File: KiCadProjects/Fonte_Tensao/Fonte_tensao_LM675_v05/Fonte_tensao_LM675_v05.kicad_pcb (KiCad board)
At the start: 2 copper layers, 90 x 100 mm, 33 parts, among them J1 alimentacao analogica, J2 sinais analogicos, J3 comunicacao / sinais digitais, J4 Barrel_Jack, U1 L7809, U2 LM7909_TO220, U3 LM675, U4 L7805, U5 L7905, U6 LM1117T-3.3

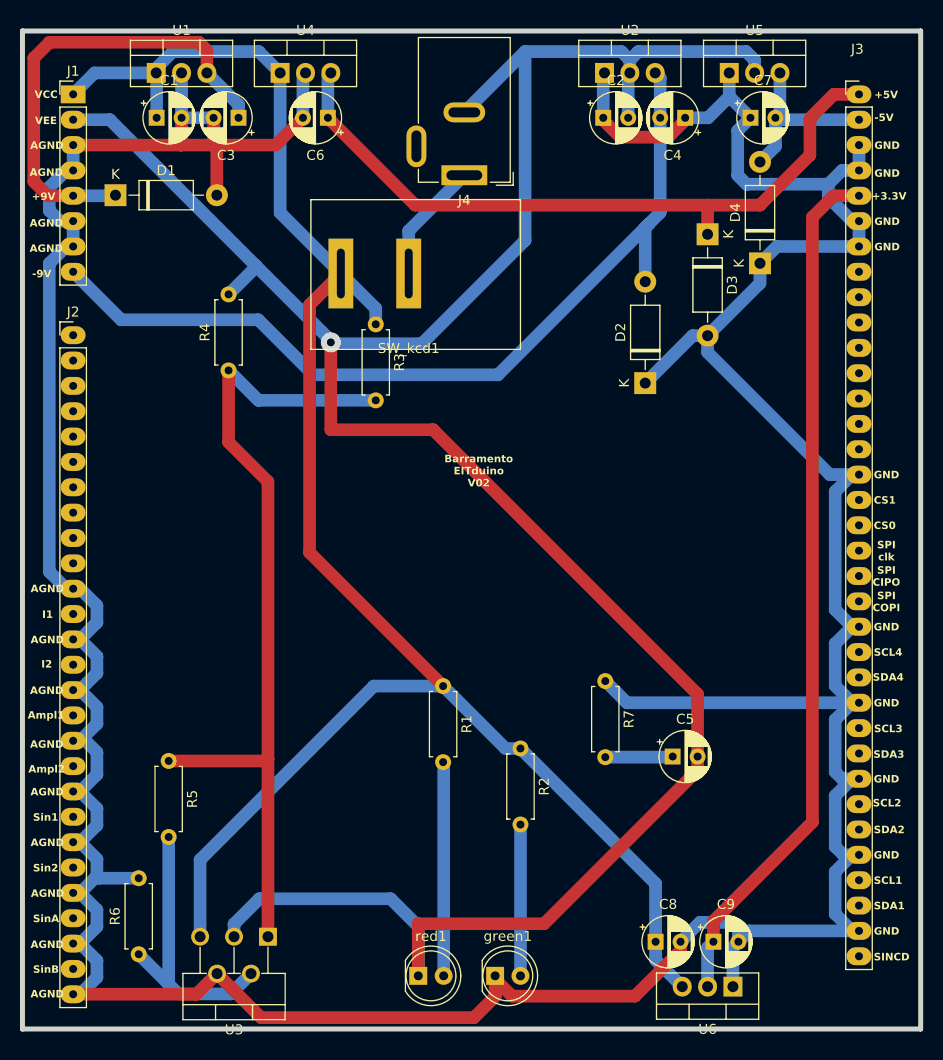
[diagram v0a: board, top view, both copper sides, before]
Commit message: versao para fabricacao jlcpcb revisao Gustavo
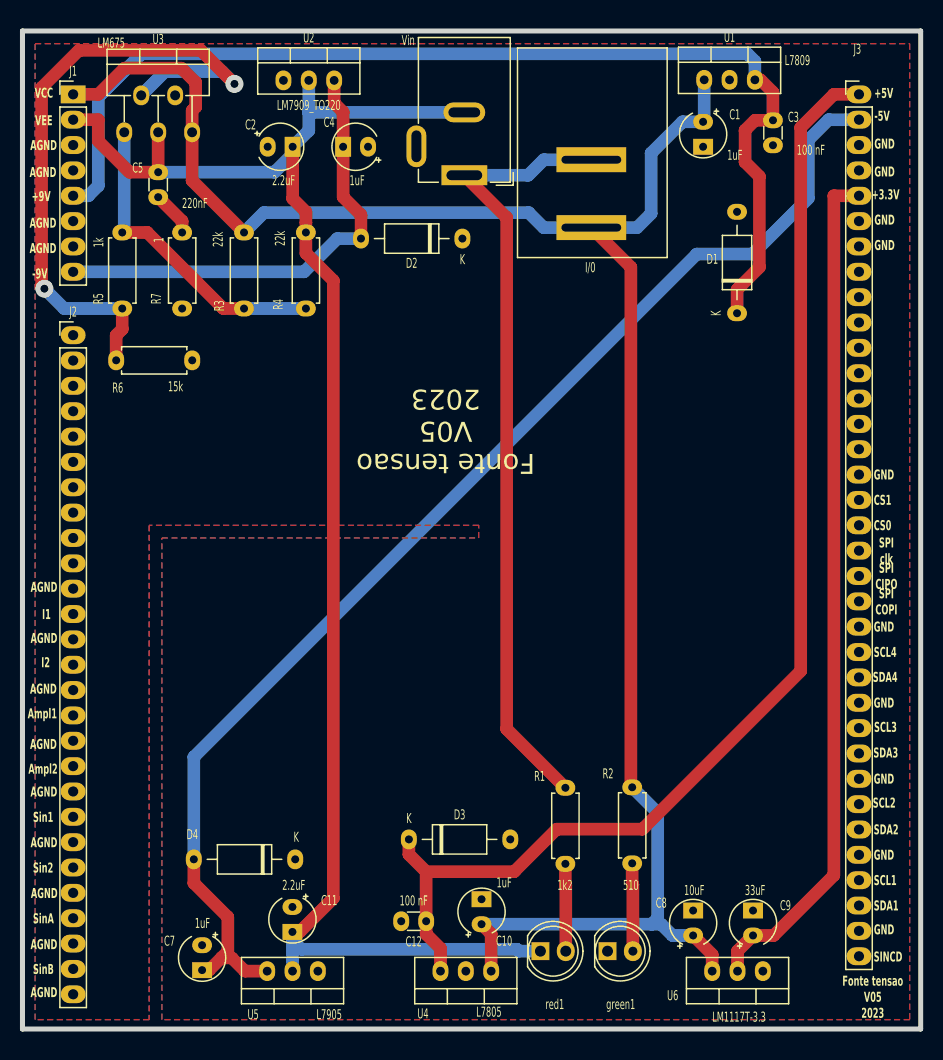
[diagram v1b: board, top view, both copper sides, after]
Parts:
- removed C6: 1uF, Capacitor_THT:CP_Radial_D5.0mm_P2.50mm
- added C10: 1uF, Capacitor_THT:CP_Radial_Tantal_D4.5mm_P2.50mm, F.Cu at (147.6, 140.3)
- added C11: 2.2uF, Capacitor_THT:CP_Radial_Tantal_D4.5mm_P2.50mm, F.Cu at (128.7, 138.6)
- added C12: 100 nF, Capacitor_THT:C_Disc_D3.0mm_W1.6mm_P2.50mm, F.Cu at (142.1, 140.0)
- C1: value 3.3uF -> 1uF; footprint Capacitor_THT:CP_Radial_D5.0mm_P2.50mm -> Capacitor_THT:CP_Radial_Tantal_D4.5mm_P2.50mm
- C2: value 22uF -> 2.2uF; footprint Capacitor_THT:CP_Radial_D5.0mm_P2.50mm -> Capacitor_THT:CP_Radial_Tantal_D4.5mm_P2.50mm
- C3: value 1uF -> 100 nF; footprint Capacitor_THT:CP_Radial_D5.0mm_P2.50mm -> Capacitor_THT:C_Disc_D3.0mm_W1.6mm_P2.50mm
- C4, C7: footprint Capacitor_THT:CP_Radial_D5.0mm_P2.50mm -> Capacitor_THT:CP_Radial_Tantal_D4.5mm_P2.50mm
- C5: value 2.2uF -> 220nF; footprint Capacitor_THT:CP_Radial_D5.0mm_P2.50mm -> Capacitor_THT:C_Disc_D3.0mm_W1.6mm_P2.50mm
- C8: value 100uF -> 10uF; footprint Capacitor_THT:CP_Radial_D5.0mm_P2.50mm -> Capacitor_THT:CP_Radial_Tantal_D4.5mm_P2.50mm
- C9: value 100uF -> 33uF; footprint Capacitor_THT:CP_Radial_D5.0mm_P2.50mm -> Capacitor_THT:CP_Radial_Tantal_D4.5mm_P2.50mm
- I/0: renamed from SW_kcd1; value chave_gangorra_2_pinos -> Vin
- Vin: renamed from J4; value Barrel_Jack -> Vin
- moved C7 99.5 mm to (119.6, 142.4), turned to -90 degrees
- moved U5 99.0 mm to (131.2, 145.0), turned to 180 degrees
- moved U4 92.5 mm to (148.6, 145.0), turned to 180 degrees
- moved U3 81.9 mm to (111.8, 61.0), turned to 0 degrees
- moved C5 76.2 mm to (115.2, 67.5), turned to 90 degrees
- moved D4 75.7 mm to (128.9, 133.8), turned to 180 degrees
- moved D3 67.6 mm to (140.3, 131.8), turned to 0 degrees
- moved D1 63.4 mm to (173.2, 79.1), turned to 90 degrees
- moved R6 59.6 mm to (111.0, 83.8), turned to 0 degrees
- moved R7 56.5 mm to (117.6, 78.6), turned to 90 degrees
- moved U1 54.9 mm to (169.9, 55.7)
- moved C1 54.8 mm to (169.8, 59.9), turned to -90 degrees
- moved C3 53.6 mm to (176.8, 59.8), turned to -90 degrees
- moved R5 53.2 mm to (111.6, 71.0)
- moved C2 33.7 mm to (126.2, 62.4)
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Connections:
- I/0 pad 1: Net-(J4-Pad1) -> Vin
- R1 pad 1: VCC -> Vin
- Vin pad 1: Net-(J4-Pad1) -> Vin
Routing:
- net Earth: track 447.4 -> 0.00 mm
- net -5V: track 18.2 -> 125.9 mm
- net VEE: track 252.2 -> 166.4 mm, vias 1 -> 0
- net Vin: track 0.00 -> 78.9 mm
- net +9V: track 47.6 -> 109.8 mm
- net Net-(U3-+): track 84.4 -> 31.7 mm
- net +5V: track 71.1 -> 122.0 mm
- net -9V: track 90.0 -> 47.2 mm
- net Net-(U3--): track 28.5 -> 67.4 mm, vias 0 -> 2
- net Net-(red1-A): track 21.4 -> 8.77 mm
- net Net-(J4-Pad1): track 12.2 -> 0.00 mm
- net VCC: track 185.7 -> 194.9 mm
- net Net-(green1-A): track 15.2 -> 8.83 mm
- net Net-(C5-Pad1): track 6.77 -> 4.53 mm
- net +3.3V: track 87.0 -> 85.4 mm
- added copper zone on B.Cu, net Earth
- added copper zone on F.Cu, net Earth
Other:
- board text added: "Fonte tensao V05 2023"
- board text removed: "Barramento EITduino V02"
